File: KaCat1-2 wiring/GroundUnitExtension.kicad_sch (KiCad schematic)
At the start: 10 parts, among them U2 OK, U3 Up, U4 Down

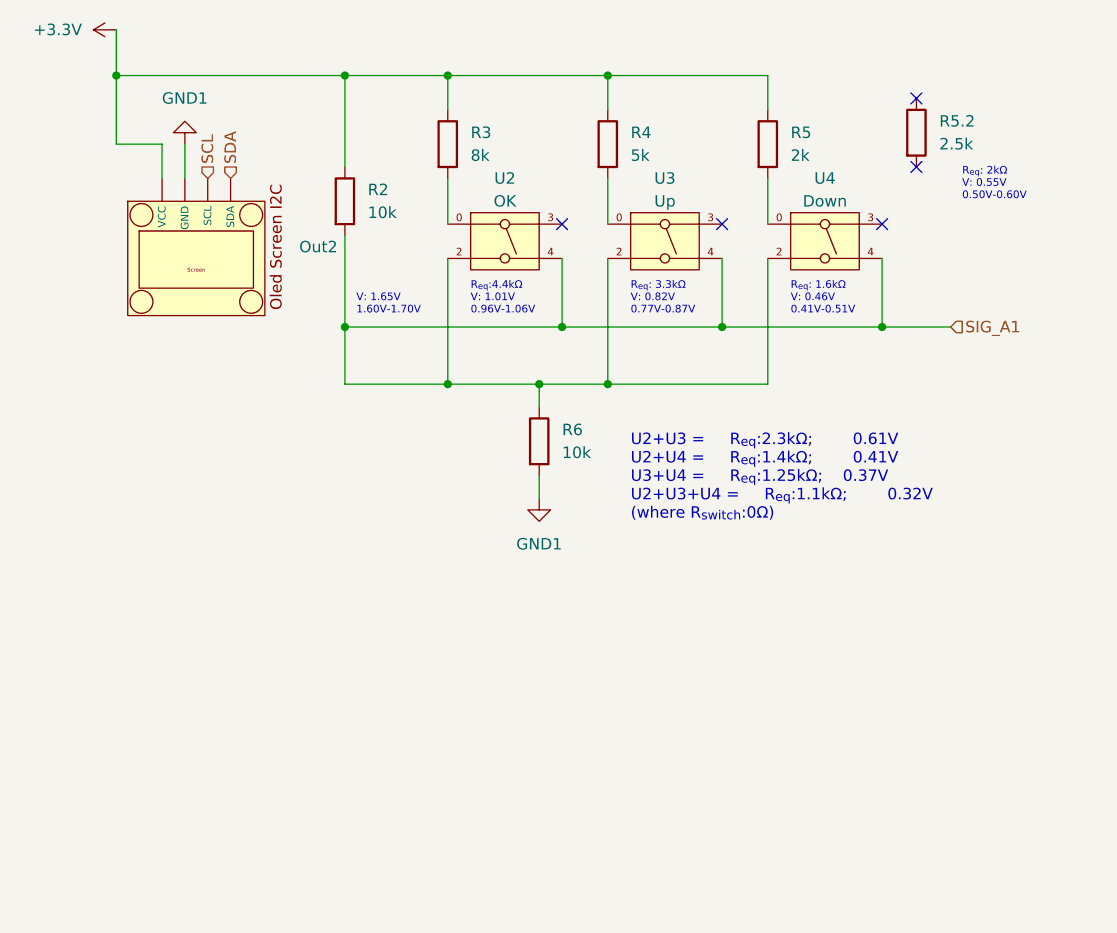
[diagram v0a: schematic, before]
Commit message: Add files via upload
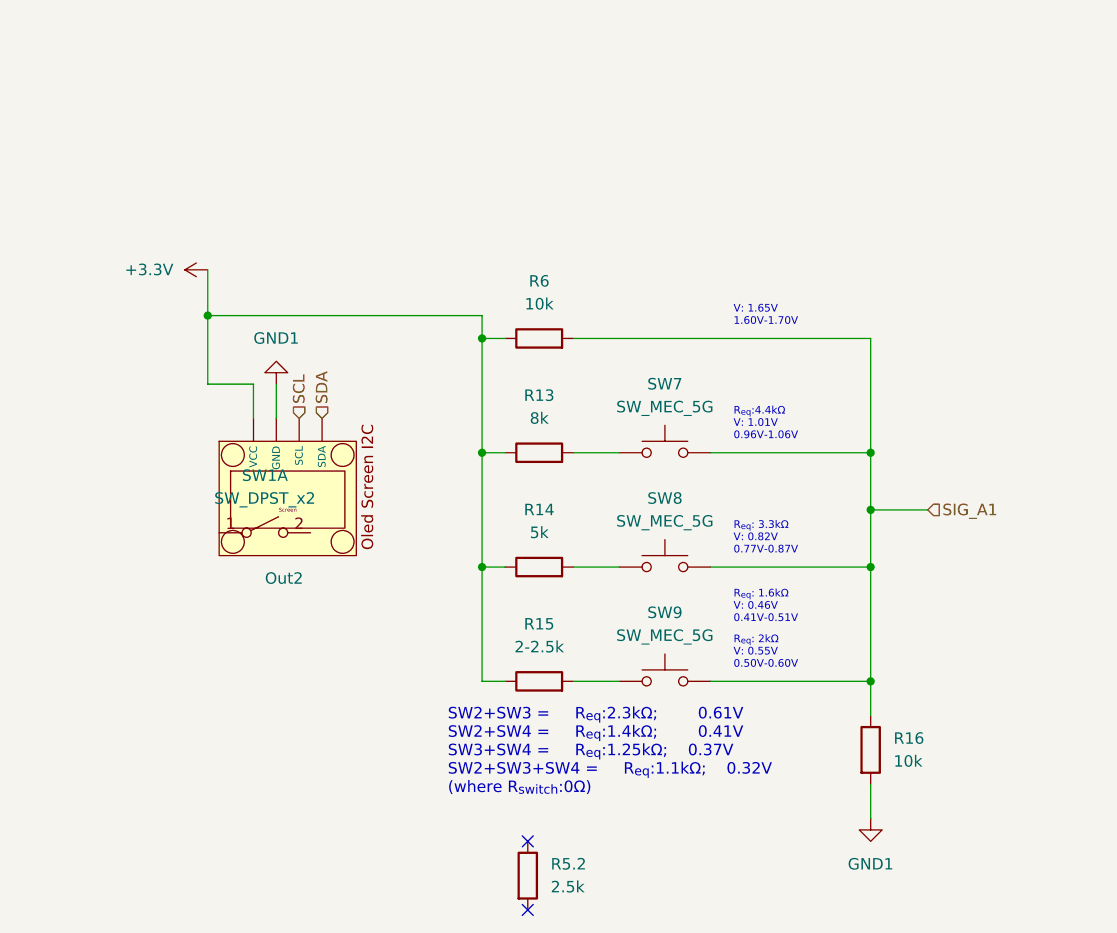
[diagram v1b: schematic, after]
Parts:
- removed R2: 10k, symbol Device:R
- removed R3: 8k, symbol Device:R
- removed R4: 5k, symbol Device:R
- removed R5: 2k, symbol Device:R
- removed U2: OK, symbol Objects:Button_Typ.0
- removed U3: Up, symbol Objects:Button_Typ.0
- removed U4: Down, symbol Objects:Button_Typ.0
- added R13: 8k, symbol Device:R
- added R14: 5k, symbol Device:R
- added R15: 2-2.5k, symbol Device:R
- added R16: 10k, symbol Device:R
- added SW1: SW_DPST_x2, symbol Switch:SW_DPST_x2
- added SW7, SW8, SW9: SW_MEC_5G, symbol Switch:SW_MEC_5G
- R5.2: now left out of the parts list
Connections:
- net +3.3V: now also R6.1, R13.1, R14.1, R15.1
- net GND1: now also R16.2; no longer R6.2
- net SIG_A1: now also R6.2, R16.1, SW7.3 (B), SW7.4 (B), SW8.3 (B), SW8.4 (B), SW9.3 (B), SW9.4 (B); no longer R6.1
- new net: R14.2, SW8.1 (A), SW8.2 (A)
- new net: R15.2, SW9.1 (A), SW9.2 (A)
- new net: R13.2, SW7.1 (A), SW7.2 (A)
- no-connect marks 5 -> 2
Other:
- note added: "SW2+SW3 = R_{eq}:2.3kΩ; 0.61V SW2+SW4 = R_{eq}:1.4kΩ; 0.41V SW3+SW4 = R_{eq}:1.25kΩ; 0.37V SW2+SW3+SW4 = R_{eq}:1.1kΩ; 0.32V (where R_{switch}:0Ω)"
- note removed: "U2+U3 = R_{eq}:2.3kΩ; 0.61V U2+U4 = R_{eq}:1.4kΩ; 0.41V U3+U4 = R_{eq}:1.25kΩ; 0.37V U2+U3+U4 = R_{eq}:1.1kΩ; 0.32V (where R_{switch}:0Ω)"
